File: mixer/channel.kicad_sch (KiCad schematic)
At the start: 38 parts, among them J7 CHANNEL_IN, J8 AVR-ISP-6, Q1 NMOS, SW1 AUX_PRE_POST_FADER_SLIDESW, SW2 MONO_PBSW, SW3 SOLO_PBSW, U10 TL074, U2 TL074, U3 DG403, U4 TL074, U5 TL074, U6 TL074, U7 TL074, U8 TL074, U9 ATtiny85-20S

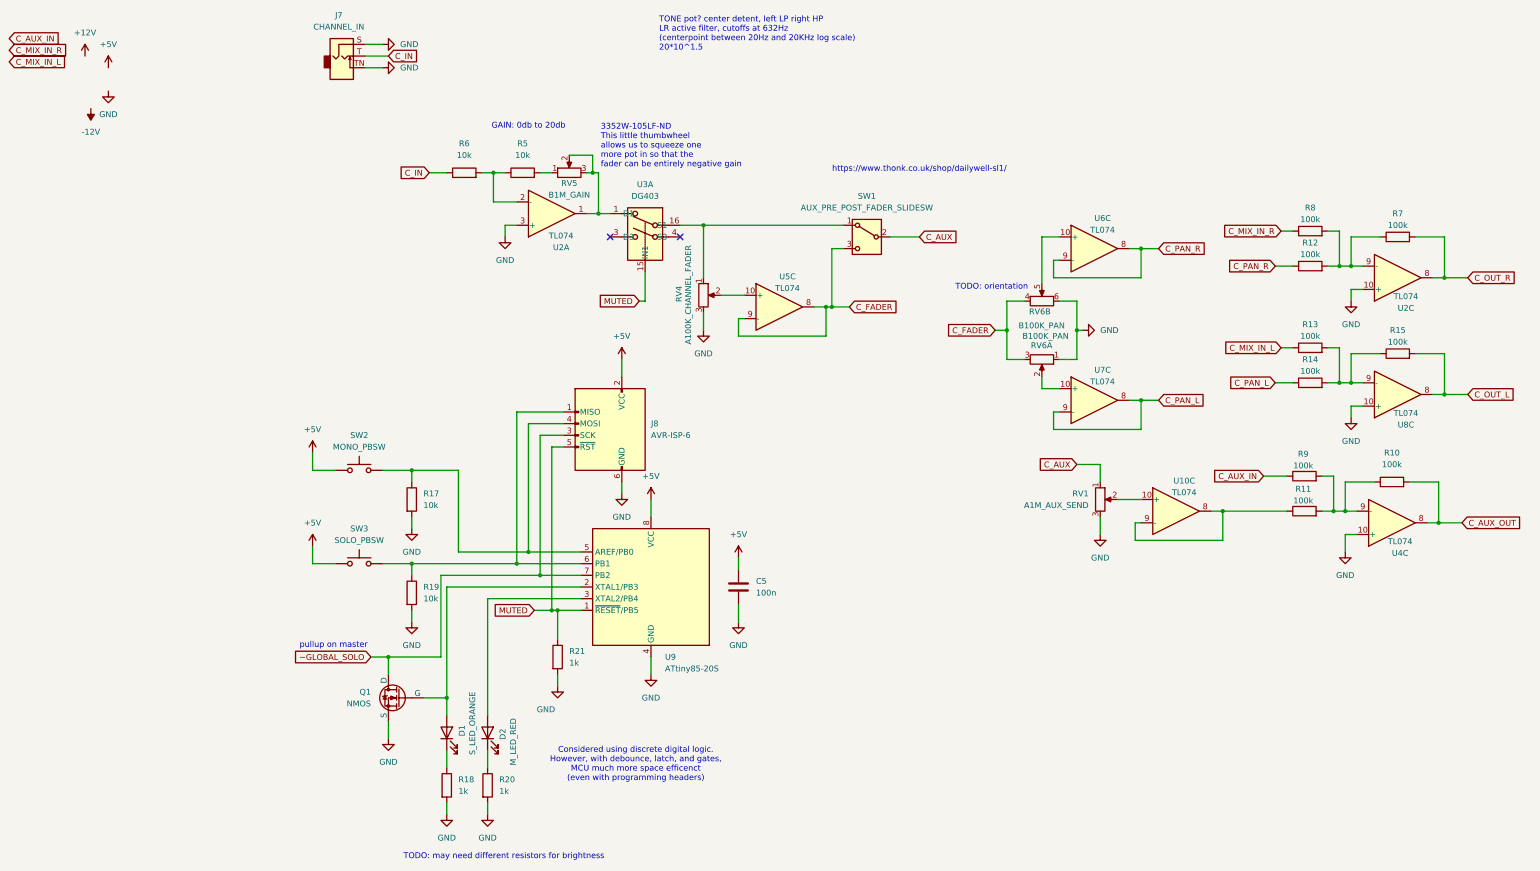
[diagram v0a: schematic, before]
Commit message: 2 channel chain
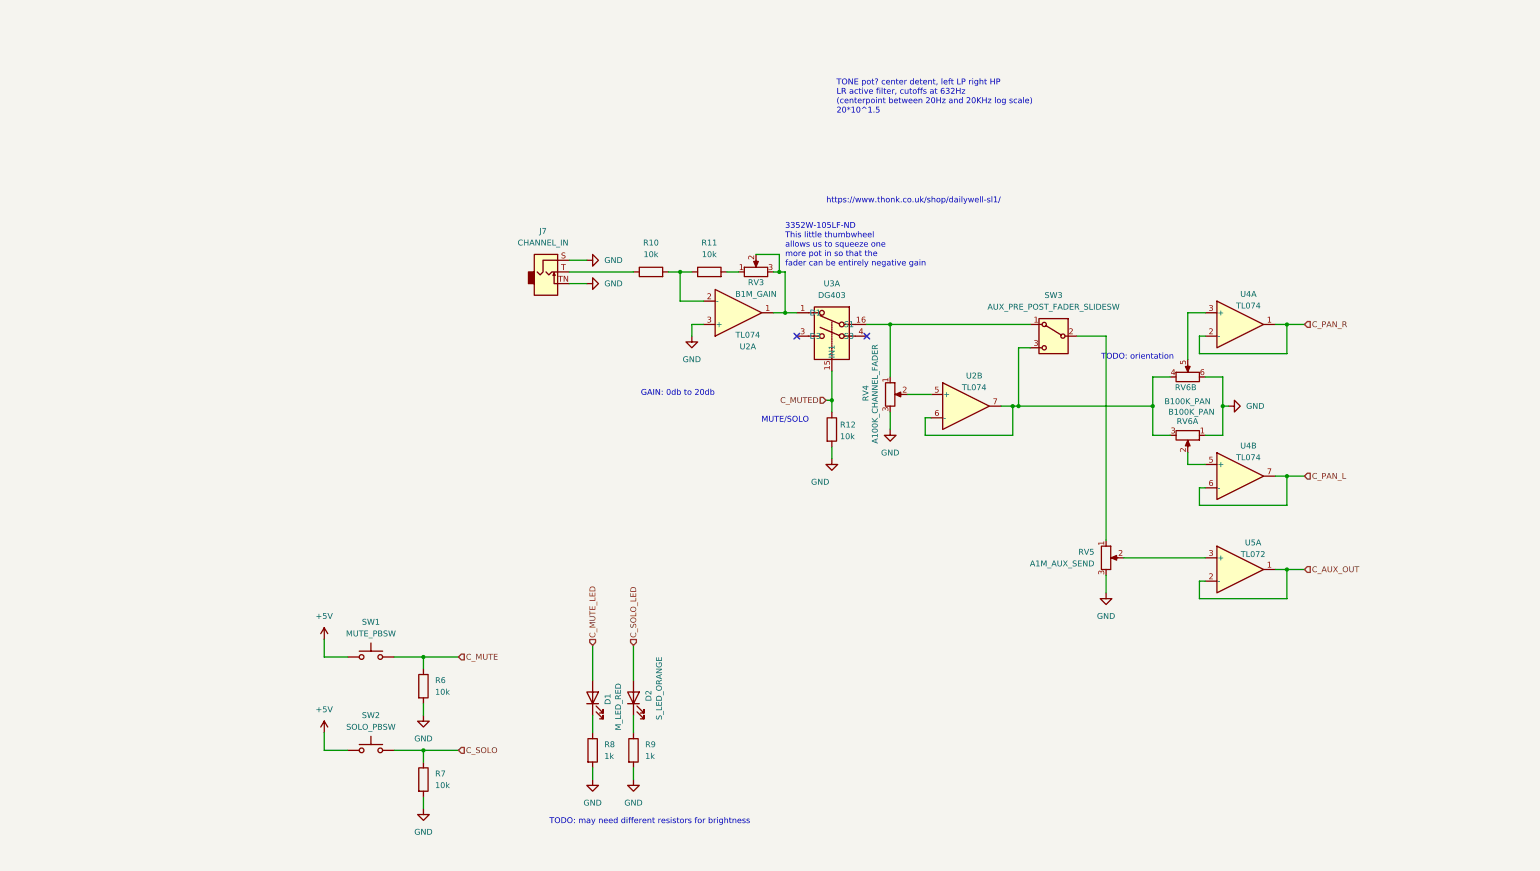
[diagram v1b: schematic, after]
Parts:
- removed C5: 100n, symbol Device:C
- removed J8: AVR-ISP-6, symbol Connector:AVR-ISP-6
- removed Q1: NMOS, symbol Simulation_SPICE:NMOS
- removed R10, R11, R12, R13, R14, R15, R7, R8, R9: 100k, symbol Device:R
- removed U10, U4, U8: TL074, symbol Amplifier_Operational:TL074
- removed unit 3 of U2
- removed U9: ATtiny85-20S, Package_SO:SOIC-8_5.3x5.3mm_P1.27mm, symbol MCU_Microchip_ATtiny:ATtiny85-20S
- added U5: TL072, symbol Amplifier_Operational:TL072
- R12: renamed from R21; value 1k -> 10k
- SW1: renamed from SW2; value MONO_PBSW -> MUTE_PBSW
- renumbered D2 to D1, D1 to D2, R6 to R10, R5 to R11, R17 to R6, R19 to R7, R18 to R8, R20 to R9, RV5 to RV3, RV1 to RV5, SW3 to SW2, SW1 to SW3, U5 to U2, U6 to U4, U7 to U4
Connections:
- net C_AUX_OUT: now also U5.1, U5.2 (-)
- net C_PAN_L: now also U4.6 (-), U4.7; no longer U4.8, U4.9 (-)
- net C_PAN_R: now also U4.1, U4.2 (-); no longer U4.8, U4.9 (-)
- net at R8.1: now also D1.1 (K); no longer D2.1 (K)
- net C_SOLO_LED: now reaches D2.2 (A)
- net C_MUTE_LED: now reaches D1.2 (A)
- net C_MUTE: now reaches R6.1, SW1.2
- net C_SOLO: now reaches R7.1, SW2.2
- net at R9.1: now also D2.1 (K); no longer D1.1 (K)
- net at RV6.2: now also U4.5 (+); no longer U4.10 (+)
- net at RV4.2: now also U2.5 (+); no longer U2.10 (+)
- net at RV5.2: now also U5.3 (+)
- net at RV6.5: now also U4.3 (+); no longer U4.10 (+)
- net C_AUX: no longer names the net of RV5.1, SW3.2 (B)
- net C_FADER: no longer names the net of RV6.3, RV6.4, SW3.3 (C)
- net C_FADER: now also U2.6 (-), U2.7; no longer U2.8, U2.9 (-)
- net C_IN: no longer names the net of J7.T, R10.1
- net MUTED renamed C_MUTED
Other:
- note added: "MUTE/SOLO"
- note removed: "Considered using discrete digital logic. However, with debounce, latch, and gates, MCU much more space efficenct (even with programming headers)"
- note removed: "pullup on master"
- moved on the sheet: D1, D2, J7, R10, R11, R12, R6, R7, R8, R9, RV3, RV4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
